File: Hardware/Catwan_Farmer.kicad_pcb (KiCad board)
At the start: 2 copper layers, 67 x 77 mm, 56 parts, among them J1 SENSOR 1, J10 VSP, J2 SENSOR 2, J3 SENSOR 3, J4 BATT, J5 USB_B, J6 Conn_01x04, J7 DHT22, J9 SENSOR 4, SW1 SW_Push, U1 AP2114N-1.0, U2 RFM95W-915S2, U3 ATSAMD21E18A-MU, U4 MCP73831-4-OT, U5 74HC4052, Y1 32.768Khz

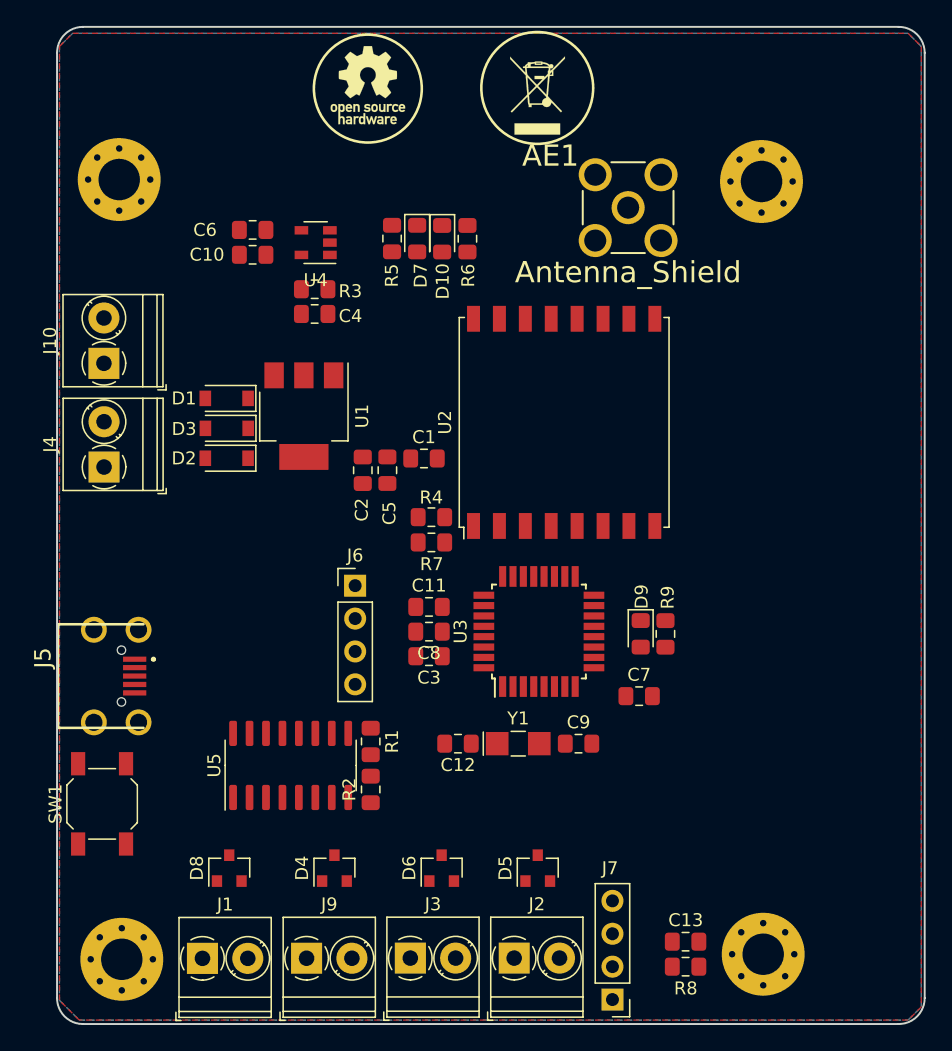
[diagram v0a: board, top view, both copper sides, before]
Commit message: Measure pcb
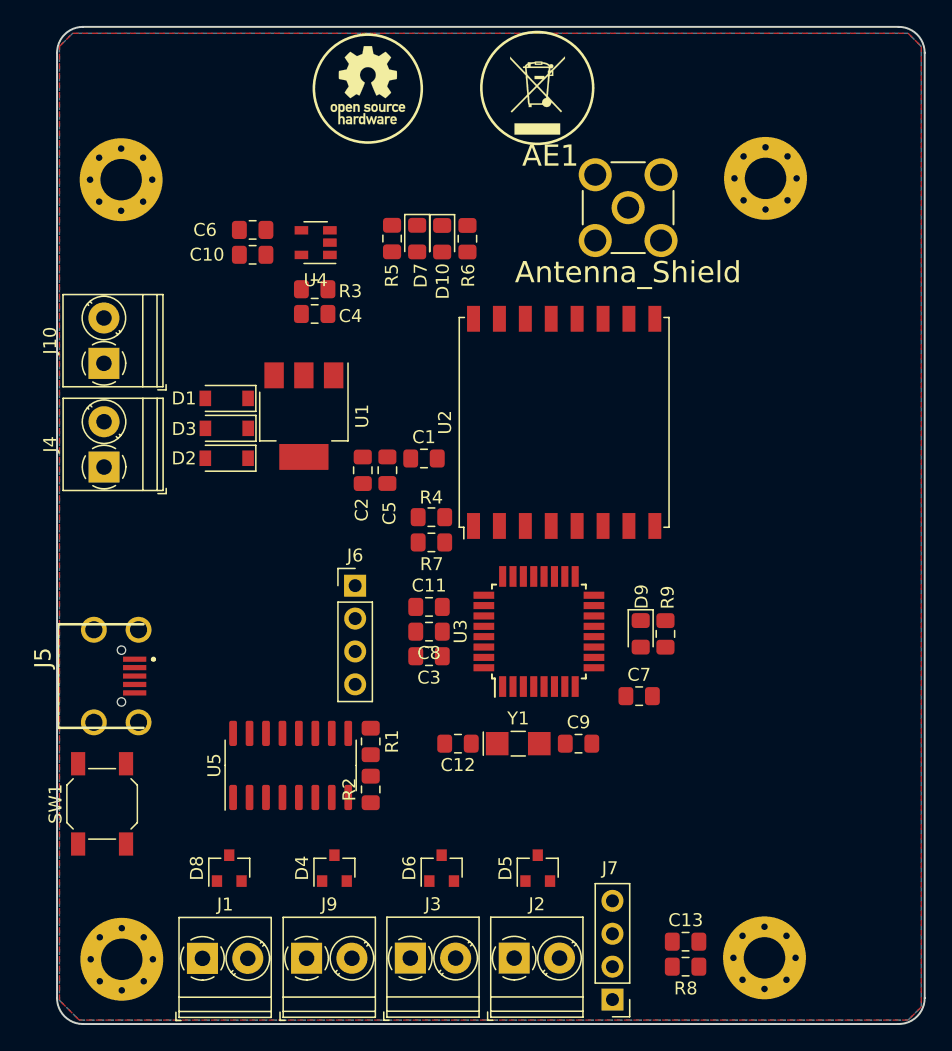
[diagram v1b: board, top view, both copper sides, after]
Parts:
- moved REF** 0.39 mm to (161.7, 42.7)
- moved REF** 0.30 mm to (161.6, 102.9)
- moved REF** 0.15 mm to (112.0, 42.8)
